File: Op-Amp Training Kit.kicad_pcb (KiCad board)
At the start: 2 copper layers, 237.7 x 121.7 mm, 145 parts, among them J1 Conn_01x04_Pin, J10 Conn_01x04_Pin, J11 Conn_01x04_Pin, J12 Conn_01x04_Pin, J13 Conn_01x04_Pin, J14 Conn_01x04_Pin, J15 Conn_01x04_Pin, J16 Conn_01x04_Pin, J17 Conn_01x04_Pin, J18 Conn_01x04_Pin, J19 Conn_01x04_Pin, J2 Conn_01x04_Pin, J20 Conn_01x04_Pin, J21 Conn_01x04_Pin, J22 Conn_01x04_Pin, J23 Conn_01x04_Pin, J24 Conn_01x04_Pin, J25 Conn_01x04_Pin, J26 Conn_01x04_Pin, J27 Conn_01x04_Pin, J28 Conn_01x04_Pin, J29 Conn_01x04_Pin, J3 Conn_01x04_Pin, J30 Conn_01x04_Pin, J31 Conn_01x04_Pin, J32 Conn_01x04_Pin, J33 Conn_01x04_Pin, J34 Conn_01x04_Pin, J35 Conn_01x04_Pin, J36 Conn_01x04_Pin, J37 Conn_01x04_Pin, J38 Conn_01x04_Pin, J39 Conn_02x04_Counter_Clockwise, J4 Conn_01x04_Pin, J40 Conn_01x04_Pin, J41 Conn_01x04_Pin, J42 Conn_01x04_Pin, J43 Conn_01x04_Pin, J44 Conn_01x04_Pin, J45 Conn_01x04_Pin, J46 Conn_01x04_Pin, J47 Conn_01x04_Pin, J48 Conn_01x04_Pin, J49 Conn_01x04_Pin, J5 Conn_01x04_Pin, J50 Conn_01x04_Pin, J51 Conn_01x02_Pin, J52 Conn_01x02_Pin, J53 Conn_01x02_Pin, J54 Conn_01x02_Pin, J55 Conn_01x02_Pin, J56 Conn_01x02_Pin, J57 Conn_01x02_Pin, J58 Conn_01x02_Pin, J59 Conn_01x04_Pin, J6 Conn_01x04_Pin, J60 Conn_01x04_Pin, J61 Conn_01x04_Pin, J62 Conn_01x04_Pin, J63 Screw_Terminal_01x03, J66 Conn_02x04_Counter_Clockwise, J67 Conn_02x04_Counter_Clockwise, J7 Conn_01x04_Pin, J8 Conn_01x04_Pin, J9 Conn_01x04_Pin, SW1 Slide Switch, SW2 Slide Switch, SW3 Slide Switch, SW4 Slide Switch, SW5 Slide Switch, SW6 Slide Switch, SW7 Slide Switch, SW8 Slide Switch, U1 LM358, U2 LM741, U3 LM741, U4 LF351N

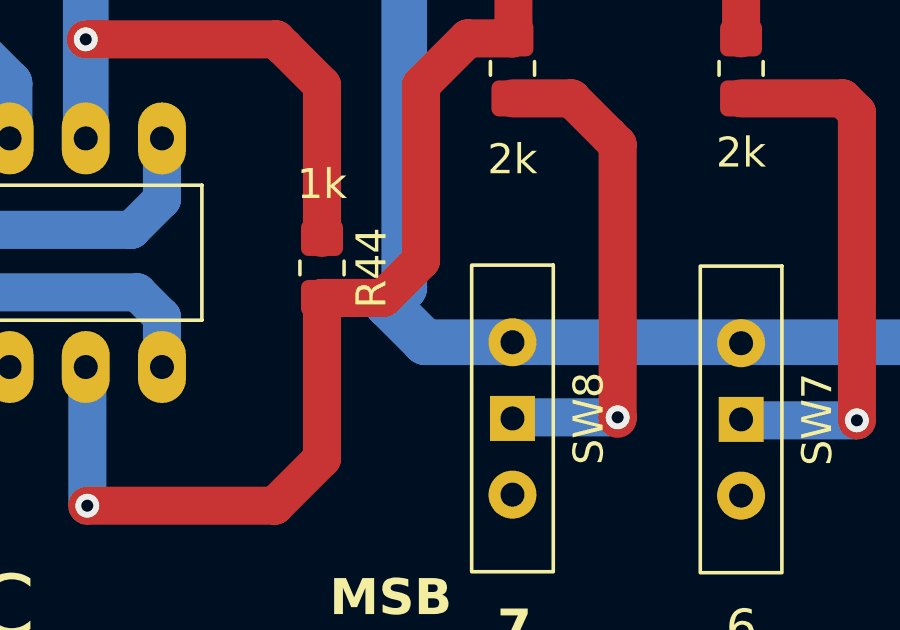
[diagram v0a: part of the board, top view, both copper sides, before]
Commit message: Updated track
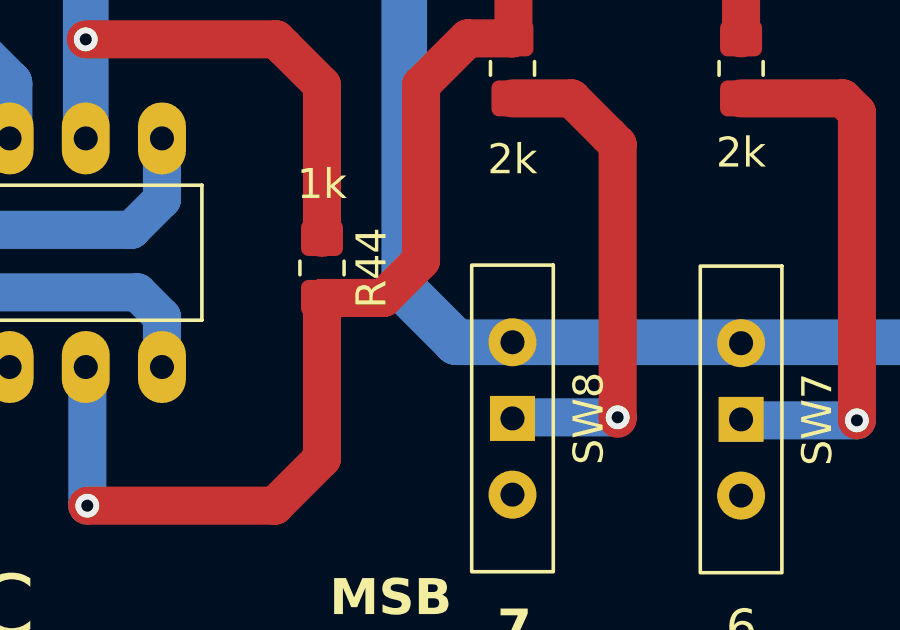
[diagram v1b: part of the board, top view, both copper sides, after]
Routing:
- net +15V: track 482.9 -> 481.8 mm
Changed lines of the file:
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@@
+	)
+	(segment
+		(start 94.14 57.34)
+		(end 92.4 55.6)
+		(width 1.524)
+		(layer "B.Cu")
+		(net 23)
+	)
+	(segment
+		(start 155.55 50.75)
+		(end 155.55 56.1844)
+		(width 1.27)
+		(layer "B.Cu")
+		(net 23)
+	)
+	(segment
+		(start 165.05 41.25)
+		(end 155.55 50.75)
+		(width 1.27)
+		(layer "B.Cu")
+		(net 23)
+	)
+	(segment
+		(start 46.2285 62.484)
+		(end 51.308 62.484)
+		(width 2.54)
+		(layer "B.Cu")
+		(net 23)
+	)
+	(segment
+		(start 65 96)
+		(end 67 98)
+		(width 2.032)
+		(layer "B.Cu")
+		(net 23)
+	)
+	(segment
+		(start 77.3684 40.0304)
+		(end 75.438 41.9608)
+		(width 1.524)
+		(layer "B.Cu")
+		(net 23)
+	)
+	(segment
+		(start 92.4052 55.5244)
+		(end 92.4052 42.7736)
+		(width 1.524)
+		(layer "B.Cu")
+		(net 23)
+	)
+	(segment
+		(start 57.15 69.85)
+		(end 57.404 70.104)
+		(width 1.524)
+		(layer "B.Cu")
+		(net 23)
+	)
+	(segment
+		(start 59 96)
+		(end 65 96)
+		(width 2.032)
+		(layer "B.Cu")
+		(net 23)
+	)
+	(segment
+		(start 58.928 62.484)
+		(end 51.308 62.484)
+		(width 2.54)
+		(layer "B.Cu")
+		(net 23)
+	)
+	(segment
+		(start 67 98)
+		(end 67 116.34)
+		(width 2.032)
+		(layer "B.Cu")
+		(net 23)
+	)
+	(segment
+		(start 57.15 63.246)
+		(end 56.388 62.484)
+		(width 2.032)
+		(layer "B.Cu")
+		(net 23)
+	)
+	(segment
+		(start 138.4616 114.2884)
+		(end 138.4616 124.1426)
+		(width 1.27)
+		(layer "B.Cu")
+		(net 23)
+	)
+	(segment
+		(start 54 91)
+		(end 59 96)
+		(width 2.032)
+		(layer "B.Cu")
+		(net 23)
+	)
+	(segment
+		(start 41.5665 57.822)
+		(end 46.2285 62.484)
+		(width 2.54)
+		(layer "B.Cu")
+		(net 23)
+	)
+	(segment
+		(start 92.4 55.6)
+		(end 92.4 55.5296)
+		(width 1.524)
+		(layer "B.Cu")
+		(net 23)
+	)
+	(segment
+		(start 54 77)
+		(end 54 91)
+		(width 2.032)
+		(layer "B.Cu")
+		(net 23)
+	)
+	(segment
+		(start 220.65 59.5)
+		(end 202.4 41.25)
+		(width 1.27)
+		(layer "B.Cu")
+		(net 23)
+	)
+	(segment
+		(start 75.438 44.9072)
+		(end 79.248 48.7172)
+		(width 1.524)
+		(layer "B.Cu")
+		(net 23)
+	)
+	(segment
+		(start 51.308 59.944)
+		(end 51.308 62.484)
+		(width 2.54)
+		(layer "B.Cu")
+		(net 23)
+	)
+	(segment
+		(start 220.65 74.17)
+		(end 220.65 59.5)
+		(width 1.27)
+		(layer "B.Cu")
+		(net 23)
+	)
+	(segment
+		(start 65.17 118.17)
+		(end 65.17 123.73)
+		(width 2.032)
+		(layer "B.Cu")
+		(net 23)
+	)
+	(segment
+		(start 57.15 75.184)
+		(end 57.15 69.85)
+		(width 2.032)
+		(layer "B.Cu")
+		(net 23)
+	)
+	(segment
+		(start 155.446 70.104)
+		(end 155.55 70)
+		(width 1.524)
+		(layer "B.Cu")
+		(net 23)
+	)
+	(segment
+		(start 96.012 57.34)
+		(end 94.14 57.34)
+		(width 1.524)
+		(layer "B.Cu")
+		(net 23)
+	)
+	(segment
+		(start 92.4052 42.7736)
+		(end 89.662 40.0304)
+		(width 1.524)
+		(layer "B.Cu")
+		(net 23)
+	)
+	(segment
+		(start 58.928 59.944)
+		(end 58.928 62.484)
+		(width 2.54)
+		(layer "B.Cu")
+		(net 23)
+	)
+	(segment
+		(start 57.15 75.184)
+		(end 55.816 75.184)
+		(width 2.032)
+		(layer "B.Cu")
+		(net 23)
 	)
 	(segment
@@
 	)
 	(segment
-		(start 155.55 50.75)
-		(end 155.55 56.1844)
-		(width 1.27)
-		(layer "B.Cu")
-		(net 23)
-	)
-	(segment
-		(start 165.05 41.25)
-		(end 155.55 50.75)
-		(width 1.27)
-		(layer "B.Cu")
-		(net 23)
-	)
-	(segment
-		(start 46.2285 62.484)
-		(end 51.308 62.484)
-		(width 2.54)
-		(layer "B.Cu")
-		(net 23)
-	)
-	(segment
-		(start 65 96)
-		(end 67 98)
-		(width 2.032)
-		(layer "B.Cu")
-		(net 23)
-	)
-	(segment
-		(start 57.15 69.85)
-		(end 57.404 70.104)
-		(width 1.524)
-		(layer "B.Cu")
-		(net 23)
-	)
-	(segment
-		(start 92.4052 55.5244)
-		(end 92.4052 42.7736)
-		(width 1.524)
-		(layer "B.Cu")
-		(net 23)
-	)
-	(segment
-		(start 59 96)
-		(end 65 96)
-		(width 2.032)
-		(layer "B.Cu")
-		(net 23)
-	)
-	(segment
-		(start 58.928 62.484)
-		(end 51.308 62.484)
-		(width 2.54)
-		(layer "B.Cu")
-		(net 23)
-	)
-	(segment
-		(start 93.1032 57.34)
-		(end 91.8464 56.0832)
-		(width 1.524)
-		(layer "B.Cu")
-		(net 23)
-	)
-	(segment
-		(start 67 98)
-		(end 67 116.34)
-		(width 2.032)
-		(layer "B.Cu")
-		(net 23)
-	)
-	(segment
-		(start 57.15 63.246)
-		(end 56.388 62.484)
-		(width 2.032)
-		(layer "B.Cu")
-		(net 23)
-	)
-	(segment
-		(start 138.4616 114.2884)
-		(end 138.4616 124.1426)
-		(width 1.27)
-		(layer "B.Cu")
-		(net 23)
-	)
-	(segment
-		(start 54 91)
-		(end 59 96)
-		(width 2.032)
-		(layer "B.Cu")
-		(net 23)
-	)
-	(segment
-		(start 41.5665 57.822)
-		(end 46.2285 62.484)
-		(width 2.54)
-		(layer "B.Cu")
-		(net 23)
-	)
-	(segment
-		(start 54 77)
-		(end 54 91)
-		(width 2.032)
-		(layer "B.Cu")
-		(net 23)
-	)
-	(segment
-		(start 220.65 59.5)
-		(end 202.4 41.25)
-		(width 1.27)
-		(layer "B.Cu")
-		(net 23)
-	)
-	(segment
-		(start 77.3684 40.0304)
-		(end 75.438 41.9608)
-		(width 1.524)
-		(layer "B.Cu")
-		(net 23)
-	)
-	(segment
-		(start 51.308 59.944)
-		(end 51.308 62.484)
-		(width 2.54)
-		(layer "B.Cu")
-		(net 23)
-	)
-	(segment
-		(start 220.65 74.17)
-		(end 220.65 59.5)
-		(width 1.27)
-		(layer "B.Cu")
-		(net 23)
-	)
-	(segment
-		(start 65.17 118.17)
-		(end 65.17 123.73)
-		(width 2.032)
-		(layer "B.Cu")
-		(net 23)
-	)
-	(segment
-		(start 57.15 75.184)
-		(end 57.15 69.85)
-		(width 2.032)
-		(layer "B.Cu")
-		(net 23)
-	)
-	(segment
-		(start 155.446 70.104)
-		(end 155.55 70)
-		(width 1.524)
-		(layer "B.Cu")
-		(net 23)
-	)
-	(segment
-		(start 58.928 59.944)
-		(end 58.928 62.484)
-		(width 2.54)
-		(layer "B.Cu")
-		(net 23)
-	)
-	(segment
-		(start 57.15 75.184)
-		(end 55.816 75.184)
-		(width 2.032)
-		(layer "B.Cu")
-		(net 23)
-	)
-	(segment
 		(start 154.3812 57.3532)
 		(end 154.368 57.34)
@@
 	)
 	(segment
-		(start 96.012 57.34)
-		(end 93.1032 57.34)
-		(width 1.524)
-		(layer "B.Cu")
-		(net 23)
-	)
-	(segment
 		(start 202.4 41.25)
 		(end 165.05 41.25)
@@
 	)
 	(segment
+		(start 75.438 41.9608)
+		(end 75.438 44.9072)
+		(width 1.524)
+		(layer "B.Cu")
+		(net 23)
+	)
+	(segment
+		(start 92.4 55.5296)
+		(end 92.4052 55.5244)
+		(width 1.524)
+		(layer "B.Cu")
+		(net 23)
+	)
+	(segment
 		(start 96.012 57.34)
 		(end 149.352 57.34)
@@
 	)
 	(segment
-		(start 75.438 44.9072)
-		(end 79.248 48.7172)
-		(width 1.524)
-		(layer "B.Cu")
-		(net 23)
-	)
-	(segment
-		(start 75.438 41.9608)
-		(end 75.438 44.9072)
-		(width 1.524)
-		(layer "B.Cu")
-		(net 23)
-	)
-	(segment
 		(start 154.368 57.34)
 		(end 149.352 57.34)
@@
 	)
 	(segment
-		(start 92.4052 42.7736)
-		(end 89.662 40.0304)
-		(width 1.524)
-		(layer "B.Cu")
-		(net 23)
-	)
-	(segment
 		(start 155.55 70)
 		(end 155.55 97.2)
@@
 		(layer "B.Cu")
 		(net 23)
-	)
-	(segment
-		(start 91.8464 56.0832)
-		(end 92.4052 55.5244)
-		(width 1.524)
-		(layer "B.Cu")
-		(net 23)
